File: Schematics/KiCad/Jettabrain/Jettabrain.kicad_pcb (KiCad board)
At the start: 2 copper layers, 38.1 x 50.8 mm, 13 parts, among them J5 Conn_01x14_Pin, J6 Conn_01x08_Pin, J7 Conn_01x01_Pin

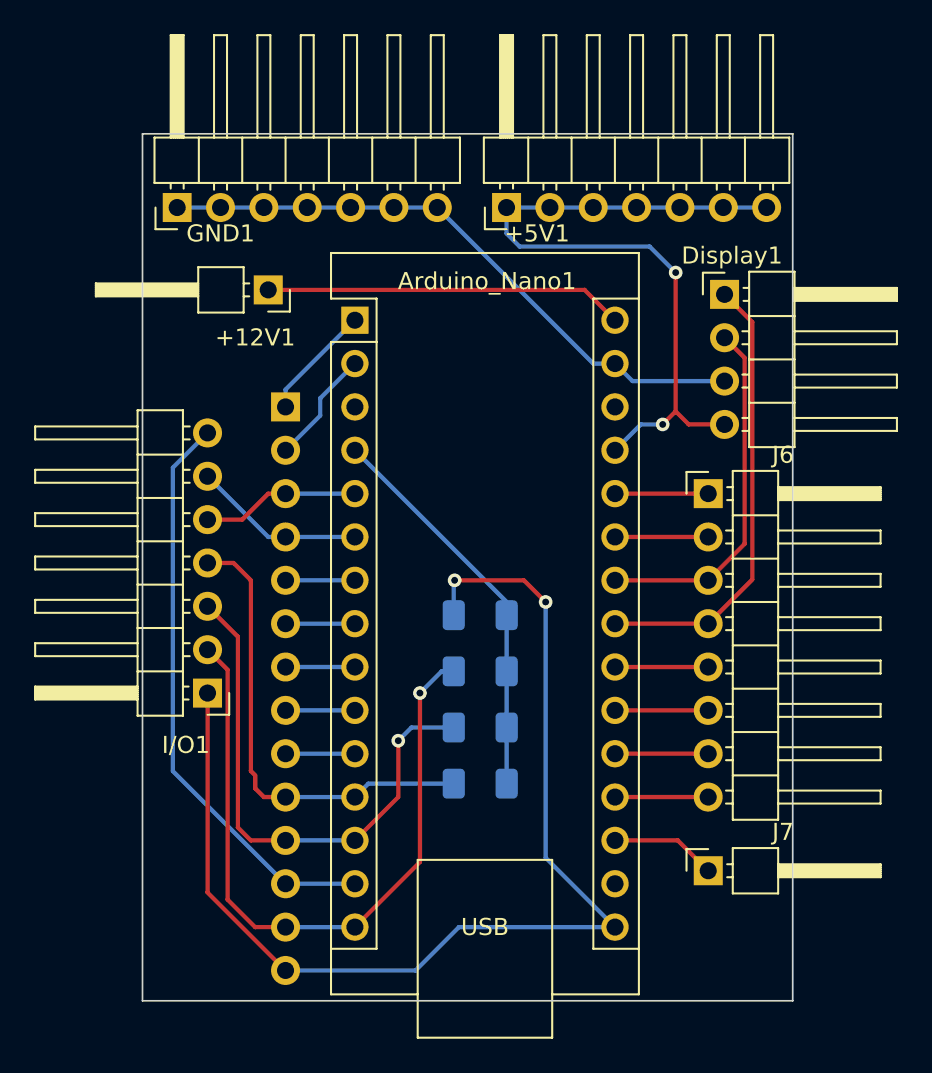
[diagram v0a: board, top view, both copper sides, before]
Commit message: PCB Updates
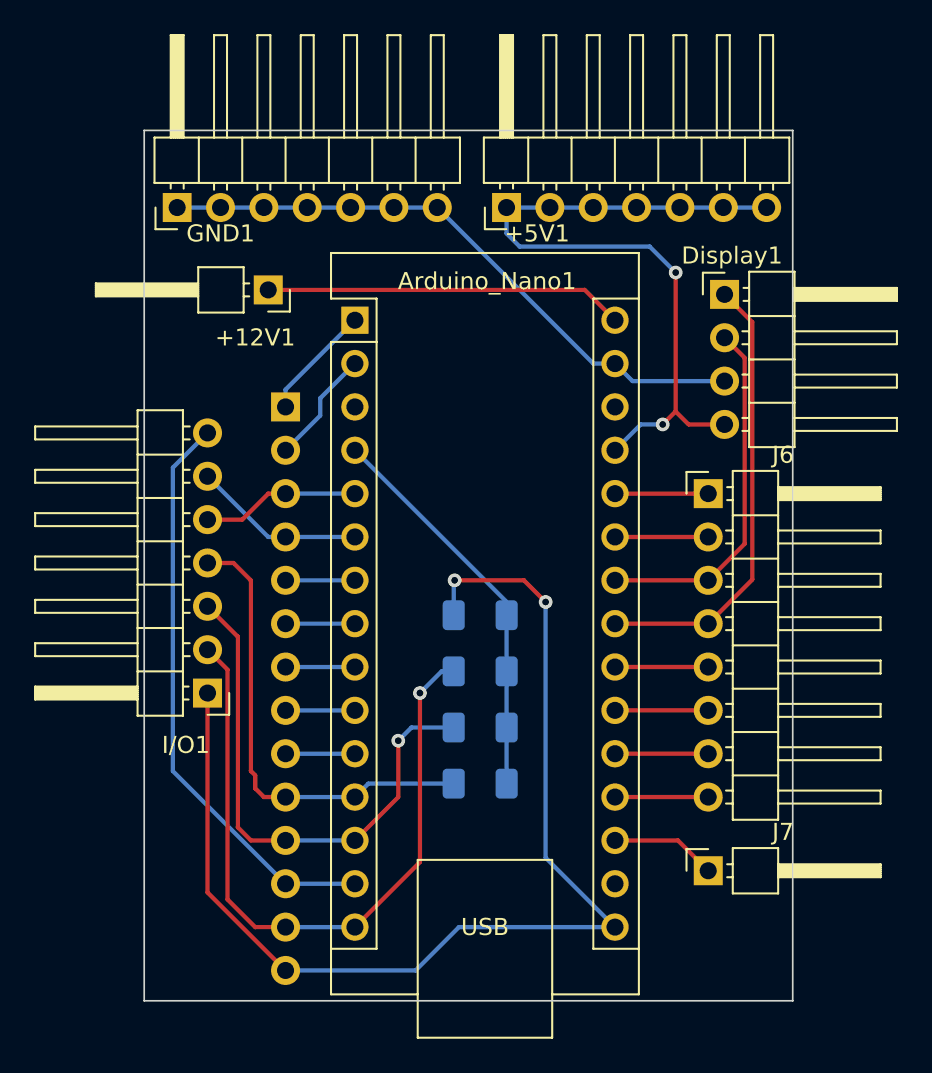
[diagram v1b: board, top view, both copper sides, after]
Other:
- board size 38.1 x 50.8 mm -> 38 x 51 mm
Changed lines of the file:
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@@
     )
   )
-  (gr_rect (start 122.174 77.47) (end 160.274 128.27)
+  (gr_rect (start 122.274 77.27) (end 160.274 128.27)
     (stroke (width 0.1) (type default)) (fill none) (layer "Edge.Cuts"))
   (gr_text "JLCJLCJLCJLC" (at 147.32 92.456) (layer "B.SilkS")
